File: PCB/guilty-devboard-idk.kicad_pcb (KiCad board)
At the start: 2 copper layers, 2 parts

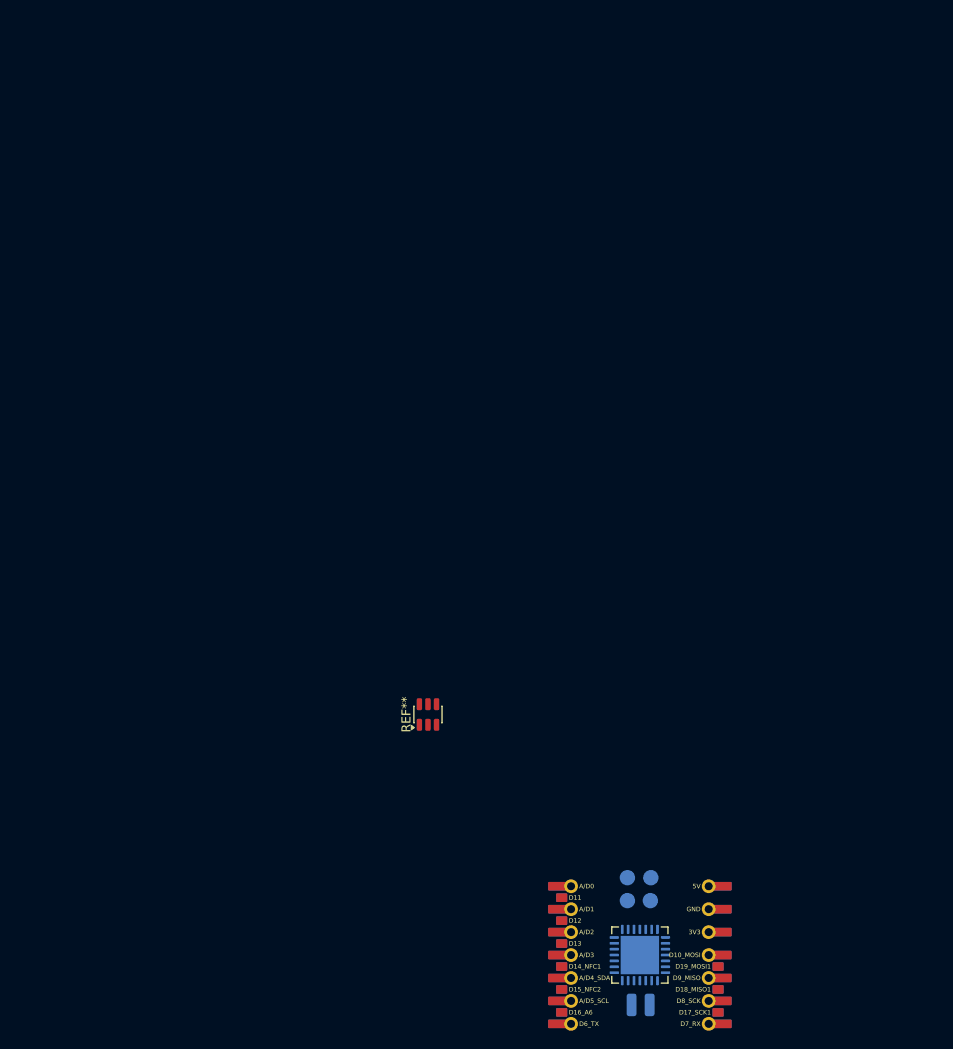
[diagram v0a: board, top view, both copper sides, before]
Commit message: terrible half done routing idk - post-decent filter routing
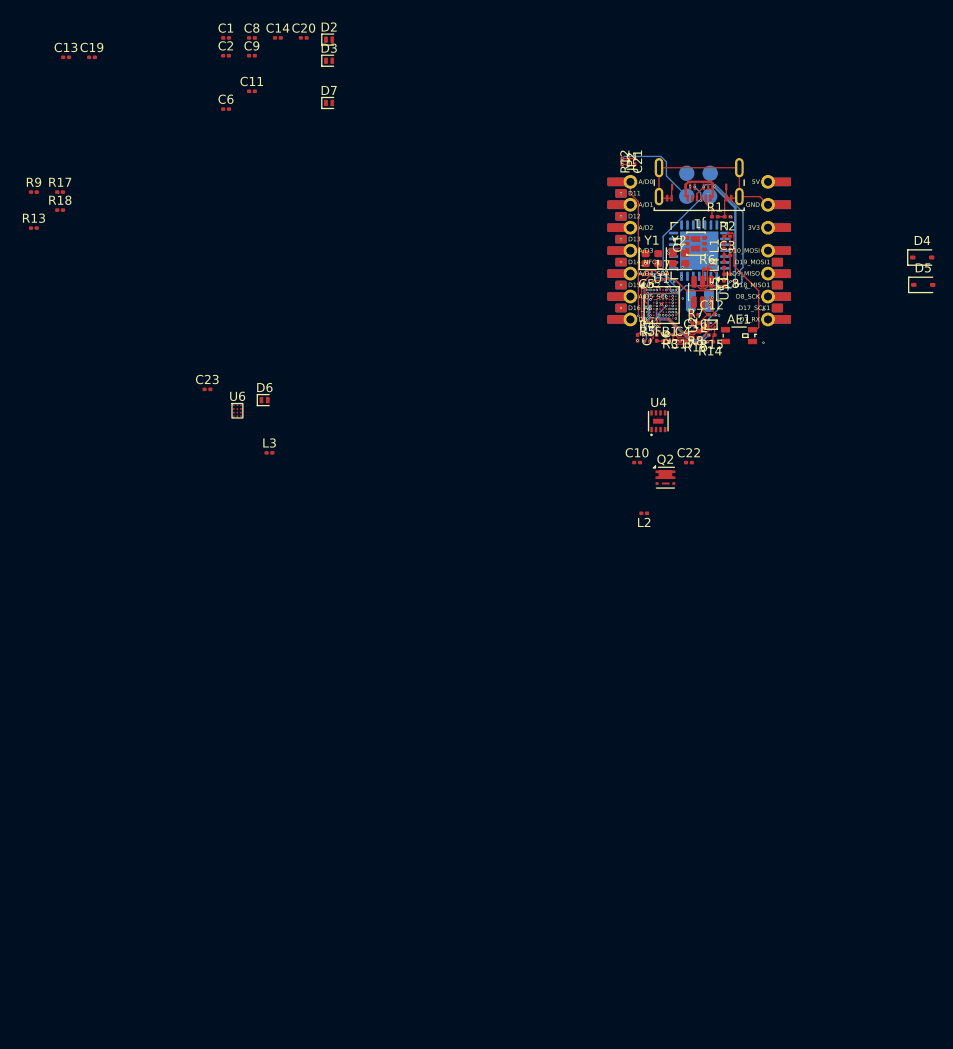
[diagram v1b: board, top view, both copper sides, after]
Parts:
- removed REF**: SOT-23-6, Package_TO_SOT_SMD:SOT-23-6
- removed REF**: Guilty Devboard Xrd pads, guilty-devboard-idk:Guilty Devboard Xrd pads
- added AE1: Antenna_Chip, PCM_marbastlib-various:2450AT18D0100001E_L, F.Cu at (120.0, 61.5)
- added C1: 10uF, Capacitor_SMD:C_0201_0603Metric, F.Cu at (63.2, 28.5)
- added C10: 4.7uF, Capacitor_SMD:C_0201_0603Metric, F.Cu at (108.7, 75.5)
- added C11: 4.7uF, Capacitor_SMD:C_0201_0603Metric, F.Cu at (66.0, 34.4)
- added C12: 0.1uF, Capacitor_SMD:C_0201_0603Metric, F.Cu at (117.0, 59.2)
- added C13: 2.2uF, Capacitor_SMD:C_0201_0603Metric, F.Cu at (45.5, 30.7)
- added C14: 4.7uF, Capacitor_SMD:C_0201_0603Metric, F.Cu at (68.9, 28.5)
- added C15: 1.5pF, Capacitor_SMD:C_0201_0603Metric, F.Cu at (118.7, 52.6)
- added C16: 22uF, Capacitor_SMD:C_0201_0603Metric, F.Cu at (115.2, 59.2)
- added C17: 4.7uF, Capacitor_SMD:C_0201_0603Metric, F.Cu at (113.8, 61.4)
- added C18: 1.2pF, Capacitor_SMD:C_0201_0603Metric, F.Cu at (118.7, 54.7)
- added C19: 22uF, Capacitor_SMD:C_0201_0603Metric, F.Cu at (48.3, 30.7)
- added C2: 100nF, Capacitor_SMD:C_0201_0603Metric, F.Cu at (63.2, 30.5)
- added C20: 22uF, Capacitor_SMD:C_0201_0603Metric, F.Cu at (71.8, 28.5)
- added C21: 100nF, Capacitor_SMD:C_0201_0603Metric, F.Cu at (107.7, 42.2)
- added C22: 1uF, Capacitor_SMD:C_0201_0603Metric, F.Cu at (114.4, 75.5)
- added C23: 0.47uF, Capacitor_SMD:C_0201_0603Metric, F.Cu at (61.1, 67.4)
- added C3: DNP, Capacitor_SMD:C_0201_0603Metric, F.Cu at (118.7, 50.5)
- added C4: 4.7uF, Capacitor_SMD:C_0201_0603Metric, F.Cu at (113.8, 62.1)
- added C5: 1.0pF, Capacitor_SMD:C_0201_0603Metric, F.Cu at (109.8, 54.7)
- added C6: 2.2uF, Capacitor_SMD:C_0201_0603Metric, F.Cu at (63.2, 36.4)
- added C7: DNP, Capacitor_SMD:C_0201_0603Metric, F.Cu at (108.8, 61.7)
- added C8: 100nF, Capacitor_SMD:C_0201_0603Metric, F.Cu at (66.0, 28.5)
- added C9: 100nF, Capacitor_SMD:C_0201_0603Metric, F.Cu at (66.0, 30.5)
- added D2: D, Diode_SMD:D_SOD-882, F.Cu at (74.6, 28.7)
- added D3: D, Diode_SMD:D_SOD-882, F.Cu at (74.6, 31.0)
- added D4: D, Diode_SMD:D_SOD-323, F.Cu at (140.3, 52.8)
- added D5: D, Diode_SMD:D_SOD-323, F.Cu at (140.4, 55.9)
- added D6: D, Diode_SMD:D_SOD-882, F.Cu at (67.4, 68.6)
- added D7: D, Diode_SMD:D_SOD-882, F.Cu at (74.6, 35.7)
- added FB1: FerriteBead, Inductor_SMD:L_0201_0603Metric, F.Cu at (111.9, 62.1)
- added J1: USB_C_Receptacle_USB2.0_16P, Connector_USB:USB_C_Receptacle_Amphenol_124019772112A, F.Cu at (115.6, 43.1)
- added JP2: Jumper_2_Bridged, Resistor_SMD:R_0201_0603Metric, F.Cu at (107.0, 42.2)
- added L1: 3.3nH, Inductor_SMD:L_0201_0603Metric, F.Cu at (118.3, 51.5)
- added L2: 2.2uH, Inductor_SMD:L_0201_0603Metric, F.Cu at (109.5, 81.2)
- added L3: 1.5uH, Inductor_SMD:L_0201_0603Metric, F.Cu at (68.0, 74.5)
- added L4: 4.7nH, Inductor_SMD:L_0201_0603Metric, F.Cu at (118.3, 53.6)
- added L5: 3.6nH, Inductor_SMD:L_0201_0603Metric, F.Cu at (118.3, 55.7)
- added L6: 4.7uH, Inductor_SMD:L_0201_0603Metric, F.Cu at (110.9, 61.7)
- added L7: 1.0nH, Inductor_SMD:L_0201_0603Metric, F.Cu at (111.6, 54.7)
- added Q1: SP2038CNQ, easyeda2kicad:PDFN-6_L2.0-W2.0-P0.65-BL-EP-1, F.Cu at (115.2, 51.3)
- added Q2: Q_PMOS, guilty-devboard-idk:Vishay_PowerPAK_SC70-6L_Single, F.Cu at (111.8, 77.2)
- added R1: 5.1k, Resistor_SMD:R_0201_0603Metric, F.Cu at (117.3, 48.3)
- added R12: 10k, Resistor_SMD:R_0201_0603Metric, F.Cu at (108.4, 42.2)
- added R13: 1M, Resistor_SMD:R_0201_0603Metric, F.Cu at (41.9, 49.6)
- added R14: 220k, Resistor_SMD:R_0201_0603Metric, F.Cu at (116.8, 62.2)
- added R15: 68k, Resistor_SMD:R_0201_0603Metric, F.Cu at (117.0, 61.4)
- added R16: 2.2, Resistor_SMD:R_0201_0603Metric, F.Cu at (115.2, 61.7)
- added R17: 200, Resistor_SMD:R_0201_0603Metric, F.Cu at (44.8, 45.6)
- added R18: 1M, Resistor_SMD:R_0201_0603Metric, F.Cu at (44.8, 47.6)
- added R2: 5.1k, Resistor_SMD:R_0201_0603Metric, F.Cu at (118.7, 48.3)
- added R3: 470k, Resistor_SMD:R_0201_0603Metric, F.Cu at (112.4, 61.4)
- added R4: 30, Resistor_SMD:R_0201_0603Metric, F.Cu at (109.8, 61.4)
- added R5: 30, Resistor_SMD:R_0201_0603Metric, F.Cu at (109.8, 62.1)
- added R6: 2k, Resistor_SMD:R_0201_0603Metric, F.Cu at (116.5, 54.1)
- added R7: 1k, Resistor_SMD:R_0201_0603Metric, F.Cu at (115.2, 60.1)
- added R8: 806k, Resistor_SMD:R_0201_0603Metric, F.Cu at (115.2, 61.0)
- added R9: 2M, Resistor_SMD:R_0201_0603Metric, F.Cu at (41.9, 45.6)
- added U1: nRF54LM20A-PAXX, PCM_nordic-lib-kicad-nrf54l:Nordic_FCCSP-98_3.67x3.85mm_Layout10x10_P0.35mm_Offcenter, F.Cu at (111.4, 58.1)
- added U2: SGM40567-4.2XG/TR, easyeda2kicad:WLCSP-6_L1.2-W0.9-R3-C2-P0.40-TL, F.Cu at (116.9, 60.3)
- added U3: Xiao nRF52840 Connectors, guilty-devboard-idk:Guilty Devboard Xrd pads, F.Cu at (115.6, 47.0)
- added U4: MIC2876-5.0YMT-TR, easyeda2kicad:UDFN-8_L2.0-W2.0-P0.50-BL-EP, F.Cu at (111.0, 71.0)
- added U5: FH9261-G3JH, Package_TO_SOT_SMD:SOT-23-6, F.Cu at (116.0, 56.6)
- added U6: BD83070GWL-E2, guilty-devboard-idk:BD83070GWL, F.Cu at (64.4, 69.8)
- added Y1: 32MHz, Crystal:Crystal_SMD_2016-4Pin_2.0x1.6mm, F.Cu at (110.3, 53.0)
- added Y2: 32.768kHz, Crystal:Crystal_SMD_2016-4Pin_2.0x1.6mm, F.Cu at (113.3, 53.0)
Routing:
- net GND: track 0.00 -> 35.1 mm, vias 0 -> 20
- net /USB_D-: track 0.00 -> 31.8 mm, vias 0 -> 4
- net VBUS: track 0.00 -> 27.4 mm, vias 0 -> 3
- net /USB_D+: track 0.00 -> 25.3 mm, vias 0 -> 3
- net /P1.03_A/D0: track 0.00 -> 20.4 mm, vias 0 -> 2
- net Net-(U1A-DECA): track 0.00 -> 16.3 mm, vias 0 -> 3
- net /P2.09_UARTE00.CTS: track 0.00 -> 15.2 mm, vias 0 -> 2
- net /P2.07_UARTE00.RXD: track 0.00 -> 14.1 mm, vias 0 -> 1
- net /P1.04_A/D1: track 0.00 -> 13.9 mm, vias 0 -> 2
- net Net-(AE1-FEED): track 0.00 -> 13.8 mm
- net /ANT: track 0.00 -> 11.9 mm
- net /RESET: track 0.00 -> 11.4 mm, vias 0 -> 2
- net /P2.10_UARTE00.RTS: track 0.00 -> 10.2 mm, vias 0 -> 2
- net /P1.01_NFC1: track 0.00 -> 9.78 mm, vias 0 -> 2
- net /P1.30_A/D4_I2C_SDA: track 0.00 -> 9.27 mm
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- added copper zone on In3.Cu, net -BATT
- added copper zone on In1.Cu, net GND
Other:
- copper layers 2 -> 6
